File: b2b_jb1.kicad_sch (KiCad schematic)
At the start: 11 parts, among them SW1 SDA02H1SBDR

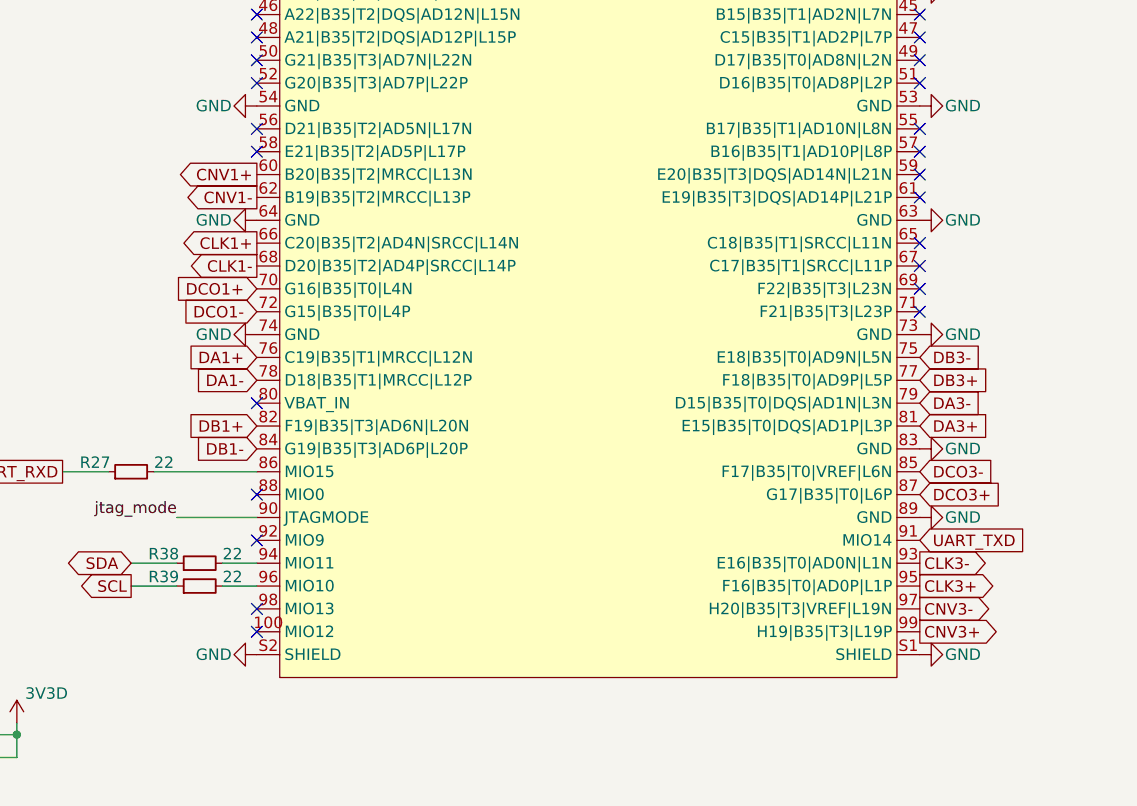
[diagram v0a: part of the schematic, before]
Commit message: edit README.md
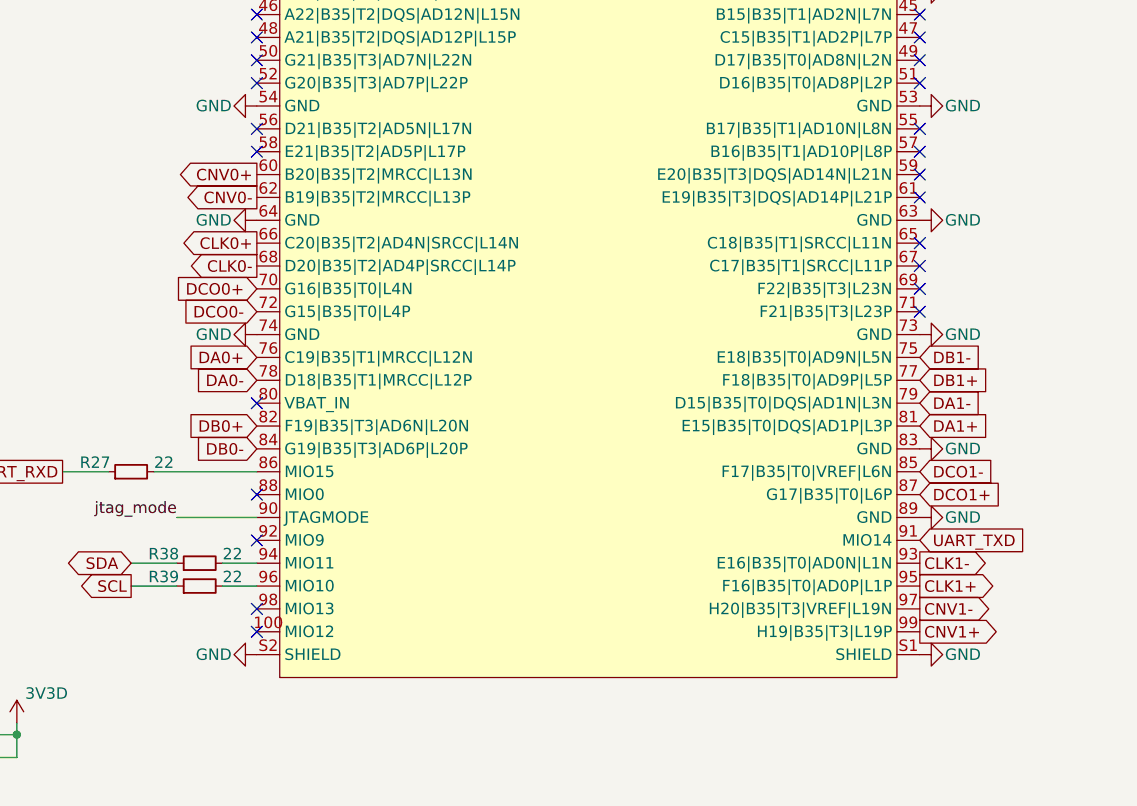
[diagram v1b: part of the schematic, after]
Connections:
- net CLK3+ is gone; now on net CLK1+: JB1.95 (F16|B35|T0|AD0P|L1P)
- net CLK3- is gone; now on net CLK1-: JB1.93 (E16|B35|T0|AD0N|L1N)
- net CNV3+ is gone; now on net CNV1+: JB1.99 (H19|B35|T3|L19P)
- net CNV3- is gone; now on net CNV1-: JB1.97 (H20|B35|T3|VREF|L19N)
- net DA3+ is gone; now on net DA1+: JB1.81 (E15|B35|T0|DQS|AD1P|L3P)
- net DA3- is gone; now on net DA1-: JB1.79 (D15|B35|T0|DQS|AD1N|L3N)
- net DB3+ is gone; now on net DB1+: JB1.77 (F18|B35|T0|AD9P|L5P)
- net DB3- is gone; now on net DB1-: JB1.75 (E18|B35|T0|AD9N|L5N)
- net DCO3+ is gone; now on net DCO1+: JB1.87 (G17|B35|T0|L6P)
- net DCO3- is gone; now on net DCO1-: JB1.85 (F17|B35|T0|VREF|L6N)
- net CLK1+: no longer JB1.66 (C20|B35|T2|AD4N|SRCC|L14N)
- net CLK1-: no longer JB1.68 (D20|B35|T2|AD4P|SRCC|L14P)
- net CNV1+: no longer JB1.60 (B20|B35|T2|MRCC|L13N)
- net CNV1-: no longer JB1.62 (B19|B35|T2|MRCC|L13P)
- net DA1+: no longer JB1.76 (C19|B35|T1|MRCC|L12N)
- net DA1-: no longer JB1.78 (D18|B35|T1|MRCC|L12P)
- net DB1+: no longer JB1.82 (F19|B35|T3|AD6N|L20N)
- net DB1-: no longer JB1.84 (G19|B35|T3|AD6P|L20P)
- net DCO1+: no longer JB1.70 (G16|B35|T0|L4N)
- net DCO1-: no longer JB1.72 (G15|B35|T0|L4P)
- new net CLK0+: JB1.66 (C20|B35|T2|AD4N|SRCC|L14N)
- new net CLK0-: JB1.68 (D20|B35|T2|AD4P|SRCC|L14P)
- new net CNV0+: JB1.60 (B20|B35|T2|MRCC|L13N)
- new net CNV0-: JB1.62 (B19|B35|T2|MRCC|L13P)
- new net DA0+: JB1.76 (C19|B35|T1|MRCC|L12N)
- new net DA0-: JB1.78 (D18|B35|T1|MRCC|L12P)
- new net DB0+: JB1.82 (F19|B35|T3|AD6N|L20N)
- new net DB0-: JB1.84 (G19|B35|T3|AD6P|L20P)
- new net DCO0+: JB1.70 (G16|B35|T0|L4N)
- new net DCO0-: JB1.72 (G15|B35|T0|L4P)
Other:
- company: (none) -> NOIRLab
- title: (none) -> 4 channel ADC Module
